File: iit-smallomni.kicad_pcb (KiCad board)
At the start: 2 copper layers, 100 x 100 mm, 83 parts, among them J1 Battery, J10 DC-Motor, J2 HC_SR04, J3 HC_SR04, J4 HC_SR04, J5 DC-Motor, J6 DC-Motor, J7 DC-Motor, J8 DC-Motor, J9 DC-Motor, Q1 2N7002, Q2 2N7002, Q3 2N7002, SW1 SW_SPDT, SW2 SW_SPDT, SW3 SW_DIP_x03, SW4 SW_Push, SW5 SW_Push, SW6 SW_Push, SW7 SW_Push, U1 NodeMCU_ESP32, U2 DSN-1504_module, U3 XL8574T, U4 XL8574T, U5 DRV-8833_module, U6 DRV-8833_module, U7 MPU-9250_IMU

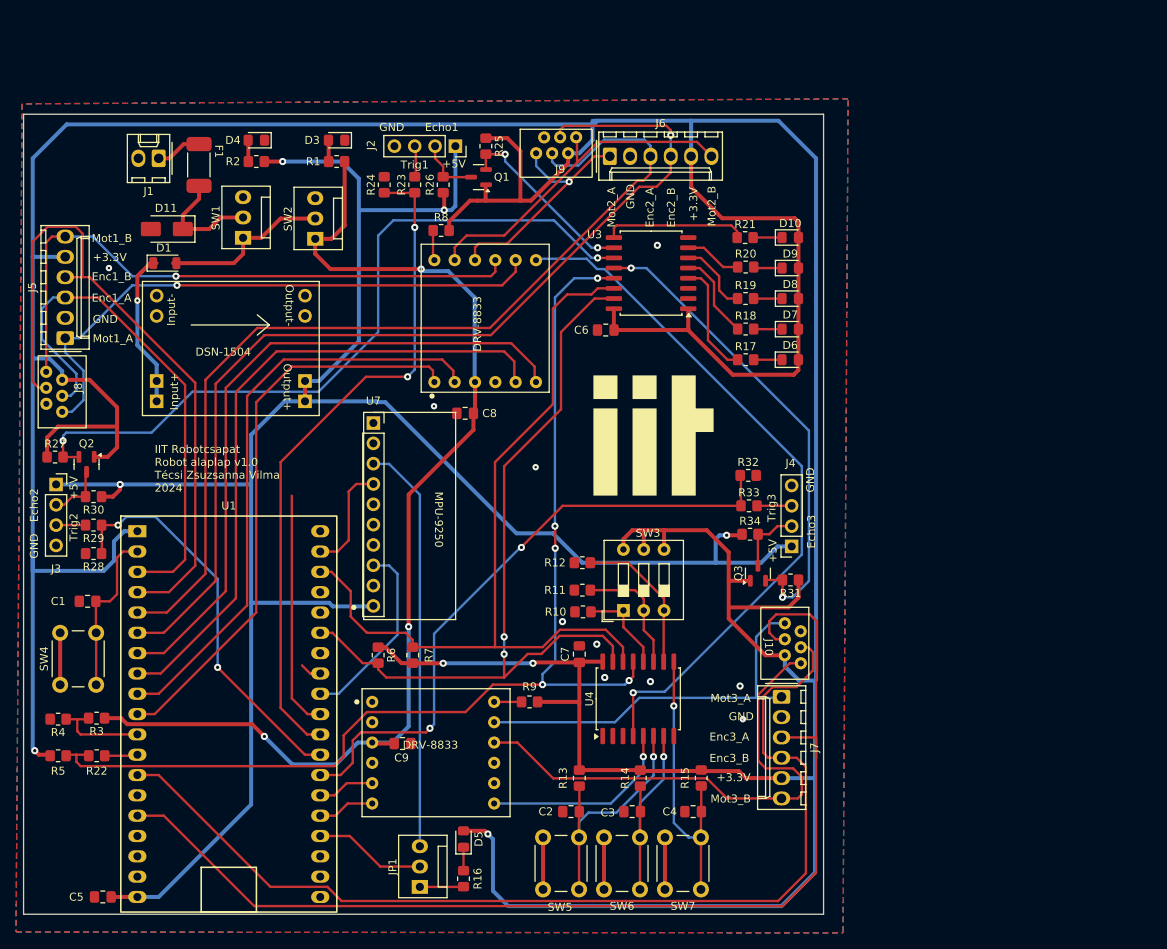
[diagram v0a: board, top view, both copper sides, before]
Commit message: Edge & basic layout
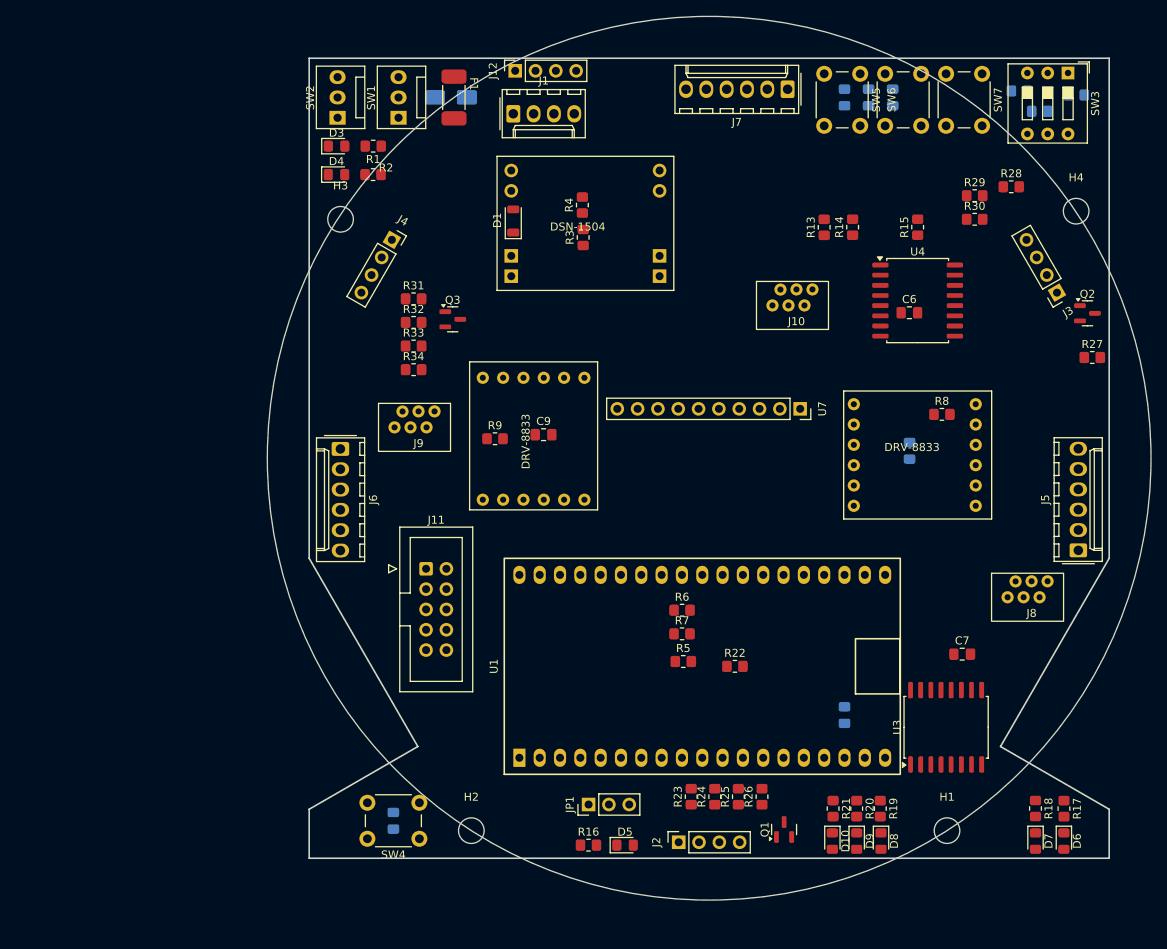
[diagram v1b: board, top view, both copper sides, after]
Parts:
- removed G***: LOGO, Onlab:IIT_logo_15x15mm
- added H1: MountingHole, MountingHole:MountingHole_3.2mm_M3, F.Cu at (229.7, 116.5)
- added H2: MountingHole, MountingHole:MountingHole_3.2mm_M3, F.Cu at (170.3, 116.5)
- added H3: MountingHole, MountingHole:MountingHole_3.2mm_M3, F.Cu at (153.9, 40.1)
- added H4: MountingHole, MountingHole:MountingHole_3.2mm_M3, F.Cu at (245.9, 39.1)
- added J11: Conn_02x05_Odd_Even, Connector_IDC:IDC-Header_2x05_P2.54mm_Vertical, F.Cu at (164.6, 83.8)
- added J12: LiPo guard, Connector_PinSocket_2.54mm:PinSocket_1x04_P2.54mm_Vertical, F.Cu at (175.8, 21.6)
- C1, C2, C3, C4, C5, C8, D11, R10, R11, R12: moved to B.Cu
- J1: footprint Connector_Molex:Molex_KK-254_AE-6410-02A_1x02_P2.54mm_Vertical -> Connector_Molex:Molex_KK-254_AE-6410-04A_1x04_P2.54mm_Vertical
- J10, J8, J9: footprint iit-smallomni:motor -> iit-smallomni:legacy-motor
- JP1: footprint Connector:FanPinHeader_1x03_P2.54mm_Vertical -> Connector_PinHeader_2.54mm:PinHeader_1x03_P2.54mm_Vertical
- moved R27 130.2 mm to (247.9, 57.4)
- moved J5 129.4 mm to (246.1, 81.5)
- moved J3 127.4 mm to (243.5, 49.3), turned to -150 degrees
- moved Q2 126.5 mm to (247.3, 51.9), turned to 0 degrees
- moved R28 123.5 mm to (237.8, 36.1), turned to 0 degrees
- moved J8 120.6 mm to (235.3, 84.4), turned to 0 degrees
- moved R29 117.6 mm to (233.2, 37.2), turned to 0 degrees
- moved R30 115.5 mm to (233.2, 40.1), turned to 0 degrees
- moved SW5 101.7 mm to (218.9, 21.9)
- moved SW6 101.7 mm to (226.5, 21.9)
- moved SW7 101.7 mm to (234.1, 21.9)
- moved C2 97.9 mm to (222.9, 24.9), turned to 90 degrees
- moved C5 95.5 mm to (216.9, 102.1), turned to 90 degrees
- moved C3 94.0 mm to (219.9, 24.9), turned to 90 degrees
- moved R4 91.8 mm to (184.2, 38.4), turned to 90 degrees
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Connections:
- J1 pad 2: GND -> /Batt_2
- R22 pad 2: Net-(U1-P14/GPIO14/ADC2_CH6) -> Net-(U1-P33/GPIO33/ADC1_CH5)
- U1 pad 10: /Mot1_DrvA -> /Mot3_EncA
- U1 pad 11: /Battery level -> Net-(JP1-C)
- U1 pad 12: Net-(U1-P14/GPIO14/ADC2_CH6) -> /JTAG_TMS
- U1 pad 13: /Mot3_EncB -> /JTAG_TDI
- U1 pad 15: /Mot3_EncA -> /JTAG_TCK
- U1 pad 23: Net-(JP1-C) -> /JTAG_TDO
- U1 pad 24: /Mot3_DrvB -> /Mot3_DrvA
- U1 pad 25: /Mot3_DrvA -> /Mot2_DrvB
- U1 pad 7: /Mot2_DrvB -> /Battery level
- U1 pad 8: /Mot2_DrvA -> Net-(U1-P33/GPIO33/ADC1_CH5)
- U1 pad 9: /Mot1_DrvB -> /Mot3_EncB
- U5 pad 1: /Mot1_DrvA -> /JTAG_TCK
- U5 pad 2: /Mot1_DrvB -> /JTAG_TDI
- U5 pad 5: /Mot2_DrvA -> /JTAG_TMS
- U6 pad 6: /Mot3_DrvB -> /JTAG_TDO
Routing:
- net +3.3V: track 627.3 -> 0.00 mm, vias 4 -> 0
- net +5V: track 263.2 -> 0.00 mm, vias 4 -> 0
- net /Mot3_EncA: track 139.9 -> 0.00 mm
- net VCC: track 138.9 -> 0.00 mm, vias 3 -> 0
- net /Interrupt: track 138.8 -> 0.00 mm, vias 5 -> 0
- net /Mot3_EncB: track 129.5 -> 0.00 mm
- net /Mot2_EncB: track 125.4 -> 0.00 mm, vias 1 -> 0
- net /Mot2_EncA: track 119.7 -> 0.00 mm
- net /I2C_SCL: track 101.7 -> 0.00 mm
- net /I2C_SDA: track 98.4 -> 0.00 mm, vias 2 -> 0
- net /UV_Trig_2: track 94.1 -> 0.00 mm, vias 2 -> 0
- net /DRV1_FAULT: track 89.0 -> 0.00 mm, vias 1 -> 0
- net /Mot1_EncB: track 85.5 -> 0.00 mm
- net /UV_Echo_1: track 84.5 -> 0.00 mm, vias 2 -> 0
- net /Mot2_DrvB: track 83.5 -> 0.00 mm
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- removed copper zone on B.Cu, net GND
- removed copper zone on F.Cu, net GND
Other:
- board size 100 x 100 mm -> 110.5 x 110.5 mm
- board text removed: "+3.3V"
- board text removed: "+5V"
- board text removed: "Echo1"
- board text removed: "Echo2"
- board text removed: "Echo3"
- board text removed: "Enc1_A"
- board text removed: "Enc1_B"
- board text removed: "Enc2_A"
- board text removed: "Enc2_B"
- board text removed: "Enc3_A"
- board text removed: "Enc3_B"
- board text removed: "GND"
- board text removed: "IIT Robotcsapat Robot alaplap v1.0 Técsi Zsuzsanna Vilma 2024"
- board text removed: "Input+"
- board text removed: "Input-"
- board text removed: "MPU-9250"
- board text removed: "Mot1_A"
- board text removed: "Mot1_B"
- board text removed: "Mot2_A"
- board text removed: "Mot2_B"
- board text removed: "Mot3_A"
- board text removed: "Mot3_B"
- board text removed: "Output+"
- board text removed: "Output-"
- board text removed: "Trig1"
- board text removed: "Trig2"
- board text removed: "Trig3"

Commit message: Routing refinement around esp and i2c
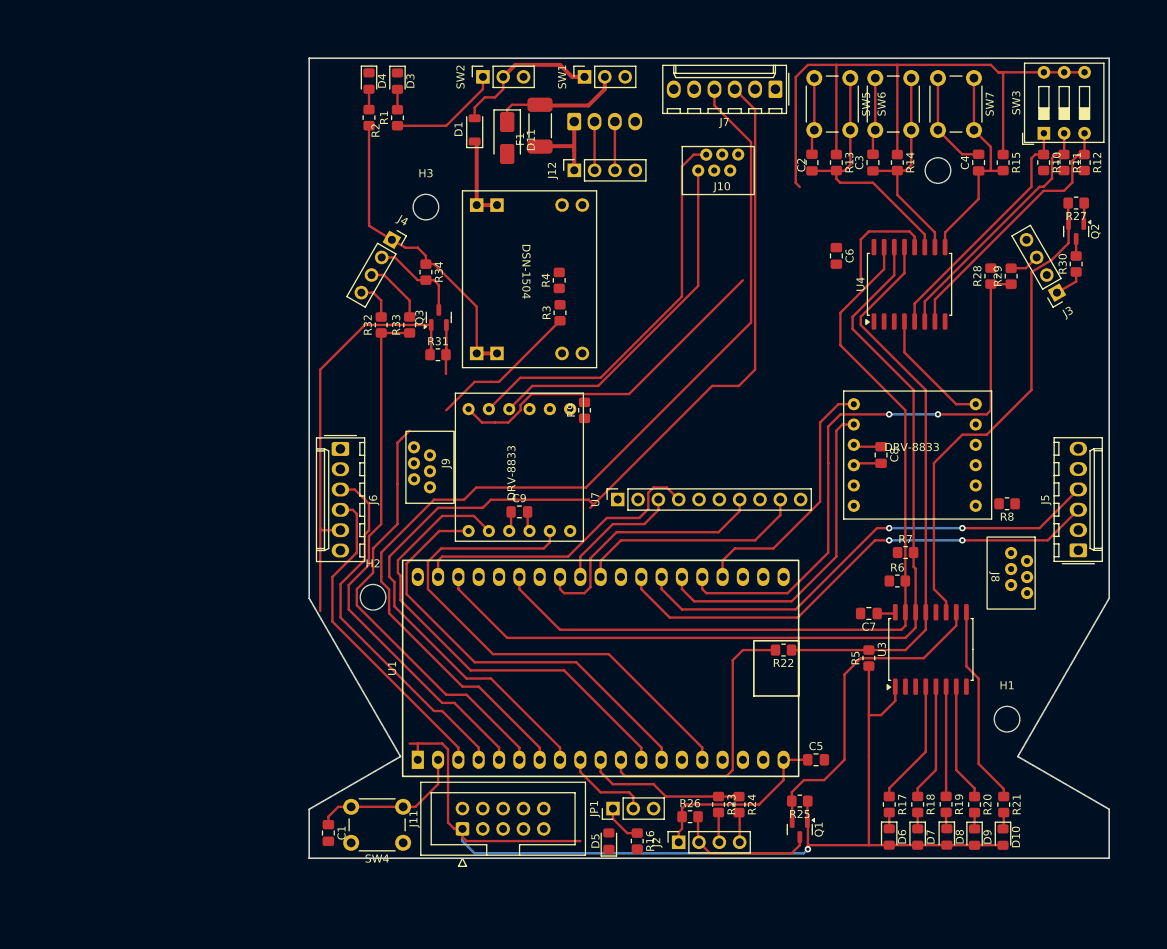
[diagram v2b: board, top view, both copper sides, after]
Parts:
- C1, C2, C3, C4, C5, C8, D11, R10, R11, R12: moved to F.Cu
- J1: moved to B.Cu
- SW1, SW2: footprint Connector:FanPinHeader_1x03_P2.54mm_Vertical -> Connector_PinSocket_2.54mm:PinSocket_1x03_P2.54mm_Vertical
- moved J11 32.8 mm to (169.2, 116.3), turned to 90 degrees
- moved H2 31.7 mm to (158.0, 87.4)
- moved R7 29.7 mm to (224.6, 81.8)
- moved R6 27.2 mm to (223.5, 85.3)
- moved U7 25.5 mm to (188.6, 75.2), turned to 90 degrees
- moved SW1 23.8 mm to (184.4, 22.3)
- moved R5 23.2 mm to (220.0, 95.0), turned to 90 degrees
- moved D6 21.8 mm to (222.5, 117.3)
- moved R17 21.8 mm to (222.5, 113.3)
- moved D10 21.3 mm to (236.7, 117.4)
- moved R21 21.3 mm to (236.8, 113.3)
- moved R27 19.4 mm to (245.9, 38.1), turned to 180 degrees
- moved J10 19.3 mm to (196.6, 31.0)
- moved SW2 18.9 mm to (171.7, 22.3)
- moved C4 18.6 mm to (233.7, 33.0)
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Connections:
- R10 pad 1: Net-(U4-P7) -> Net-(U4-P1)
- R11 pad 1: Net-(U4-P6) -> Net-(U4-P2)
- R12 pad 1: Net-(U4-P5) -> Net-(U4-P3)
- R22 pad 2: Net-(U1-P33/GPIO33/ADC1_CH5) -> Net-(U1-P27/GPIO27/ADC2_CH7)
- R8 pad 2: Net-(U5-FAULT) -> Net-(U5-SLEEP)
- R9 pad 2: Net-(U6-FAULT) -> Net-(U6-SLEEP)
- SW3 pad 1: Net-(U4-P7) -> Net-(U4-P1)
- SW3 pad 2: Net-(U4-P6) -> Net-(U4-P2)
- SW3 pad 3: Net-(U4-P5) -> Net-(U4-P3)
- U1 pad 10: /Mot3_EncA -> /UV_Echo_1
- U1 pad 11: Net-(JP1-C) -> Net-(U1-P27/GPIO27/ADC2_CH7)
- U1 pad 24: /Mot3_DrvA -> /UV_Echo_2
- U1 pad 25: /Mot2_DrvB -> /Mot1_DrvB
- U1 pad 26: /UV_Echo_3 -> /Mot1_EncB
- U1 pad 27: /UV_Echo_2 -> /Mot1_EncA
- U1 pad 28: /UV_Echo_1 -> /Mot3_DrvB
- U1 pad 3: /Mot1_EncA -> /Mot2_EncB
- U1 pad 4: /Mot1_EncB -> /Mot2_EncA
- U1 pad 5: /Mot2_EncA -> /UV_Echo_3
- U1 pad 6: /Mot2_EncB -> /Battery level
- U1 pad 7: /Battery level -> /Mot3_EncB
- U1 pad 8: Net-(U1-P33/GPIO33/ADC1_CH5) -> /Mot3_EncA
- U1 pad 9: /Mot3_EncB -> Net-(JP1-C)
- U4 pad 10: Net-(U4-P5) -> /Button_2
- U4 pad 11: Net-(U4-P6) -> /Button_1
- U4 pad 12: Net-(U4-P7) -> /DRV2_FAULT
- U4 pad 5: /DRV2_FAULT -> Net-(U4-P1)
- U4 pad 6: /Button_1 -> Net-(U4-P2)
- U4 pad 7: /Button_2 -> Net-(U4-P3)
- U5 pad 1: /JTAG_TCK -> /JTAG_TDO
- U5 pad 10: /Mot2_A -> unconnected-(U5-OUT3-Pad10)
- U5 pad 11: /Mot2_B -> unconnected-(U5-OUT4-Pad11)
- U5 pad 12: Net-(U5-FAULT) -> /DRV1_FAULT
- U5 pad 2: /JTAG_TDI -> /Mot1_DrvB
- U5 pad 5: /JTAG_TMS -> unconnected-(U5-IN3-Pad5)
- U5 pad 6: /Mot2_DrvB -> unconnected-(U5-IN4-Pad6)
- U5 pad 7: /DRV1_FAULT -> Net-(U5-SLEEP)
- U6 pad 1: unconnected-(U6-IN1-Pad1) -> /JTAG_TDI
- U6 pad 10: /Mot3_B -> /Mot3_A
- U6 pad 11: /Mot3_A -> /Mot3_B
- U6 pad 12: Net-(U6-FAULT) -> /DRV2_FAULT
- U6 pad 2: unconnected-(U6-IN2-Pad2) -> /JTAG_TMS
- U6 pad 5: /Mot3_DrvA -> /JTAG_TCK
- U6 pad 6: /JTAG_TDO -> /Mot3_DrvB
- U6 pad 7: /DRV2_FAULT -> Net-(U6-SLEEP)
- U6 pad 8: unconnected-(U6-OUT1-Pad8) -> /Mot2_B
- U6 pad 9: unconnected-(U6-OUT2-Pad9) -> /Mot2_A
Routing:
- net +3.3V: track 0.00 -> 280.9 mm, vias 0 -> 1
- net /Mot3_EncA: track 0.00 -> 128.6 mm
- net /Mot3_EncB: track 0.00 -> 124.7 mm
- net /I2C_SCL: track 0.00 -> 114.7 mm
- net /I2C_SDA: track 0.00 -> 105.4 mm
- net /UV_Echo_2: track 0.00 -> 74.8 mm, vias 0 -> 2
- net /Interrupt: track 0.00 -> 71.3 mm
- net /UV_Echo_3: track 0.00 -> 67.3 mm
- net /JTAG_TCK: track 0.00 -> 65.1 mm
- net /Mot1_EncA: track 0.00 -> 63.2 mm, vias 0 -> 2
- net /Mot1_EncB: track 0.00 -> 60.9 mm, vias 0 -> 2
- net /JTAG_TMS: track 0.00 -> 58.8 mm
- net +5V: track 0.00 -> 58.8 mm
- net /UV_Trig_2: track 0.00 -> 58.0 mm
- net /DRV2_FAULT: track 0.00 -> 56.5 mm
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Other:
- board size 110.5 x 110.5 mm -> 100 x 100 mm
